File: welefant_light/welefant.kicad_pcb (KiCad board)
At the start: 2 copper layers, 80 x 90 mm, 103 parts, among them J1 Conn_01x02, J2 Conn_02x7_Odd_Even, J3 Conn_02x6_Odd_Even, Q1 AO3401A, Q2 AO3401A, Q3 AO3401A, SW1 ON-OFF, SW2 RESET, SW3 BOOT, SW4 GPIO33, SW5 IO34, U1 RT9080-33GJ5, U2 Audio Jack PJ-324, U3 SD18OB261-060, U4 TP4056, U5 welefant, U6 128MBit Flash, U7 ESP32-S3, U8 Reset 2.8V, X1 40 MHz

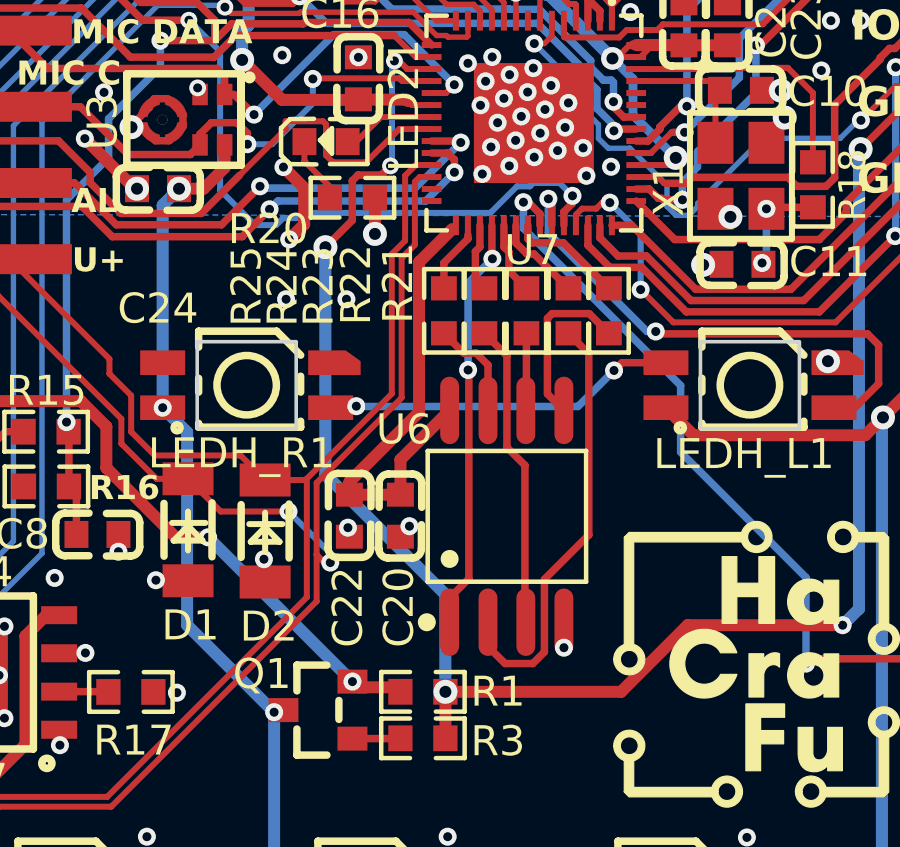
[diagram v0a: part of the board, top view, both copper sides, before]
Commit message: use S3FH4R2 / remove flash chip
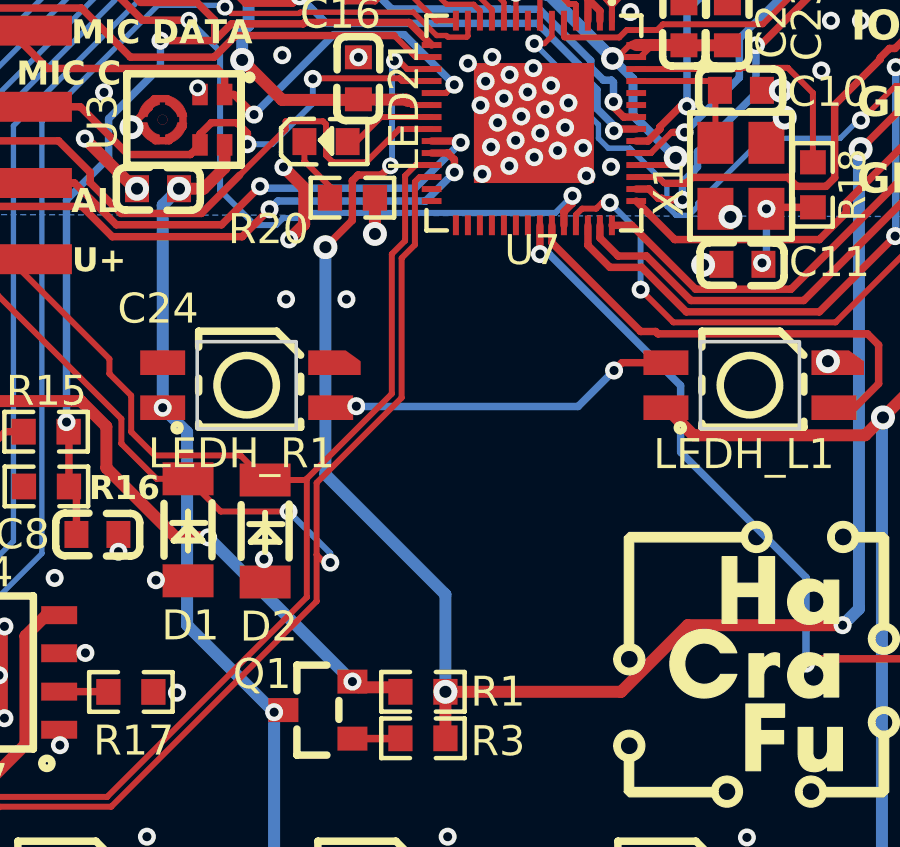
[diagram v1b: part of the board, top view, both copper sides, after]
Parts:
- removed C20: 100n, easyeda2kicad:C0603
- removed C22: 1u, easyeda2kicad:C0603
- removed R21, R22, R23, R24, R25: 0, easyeda2kicad:R0603
- removed U6: 128MBit Flash, easyeda2kicad:SOIC-8_L5.3-W5.3-P1.27-LS8.0-BL
- U7: value ESP32-S3 -> ESP32-S3FH4R2
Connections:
- U7 pad 29: /VDD_SPI -> unconnected-(U7-VDD_SPI-Pad29)
- U7 pad 30: Net-(U7-SPIHD) -> unconnected-(U7-SPIHD-Pad30)
- U7 pad 31: Net-(U7-SPIWP) -> unconnected-(U7-SPIWP-Pad31)
- U7 pad 32: /SPICS0 -> unconnected-(U7-SPICS0-Pad32)
- U7 pad 33: Net-(U7-SPICLK) -> unconnected-(U7-SPICLK-Pad33)
- U7 pad 34: Net-(U7-SPIQ) -> unconnected-(U7-SPIQ-Pad34)
- U7 pad 35: Net-(U7-SPID) -> unconnected-(U7-SPID-Pad35)
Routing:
- net /VDD_SPI: track 15.6 -> 0.00 mm
- net /SPIQ: track 14.6 -> 0.00 mm
- net /SPICS0: track 13.8 -> 0.00 mm, vias 2 -> 0
- net /SPIWP: track 10.2 -> 0.00 mm
- net /SPID: track 5.68 -> 0.00 mm
- net Net-(U7-SPID): track 3.84 -> 0.00 mm
- net /SPIHD: track 3.42 -> 0.00 mm
- net Net-(U7-SPIQ): track 2.96 -> 0.00 mm
- net /SPICLK: track 2.58 -> 0.00 mm
- net Net-(U7-SPICLK): track 2.41 -> 0.00 mm
- net Net-(U7-SPIWP): track 2.29 -> 0.00 mm
- net Net-(U7-SPIHD): track 2.12 -> 0.00 mm
- net /LED_MATRIX: track 35.7 -> 33.8 mm
- net /LED_HEAD: track 17.7 -> 16.0 mm, vias 2 -> 0
- net GND: vias 458 -> 455

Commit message: Revert "use S3FH4R2 / remove flash chip"
This reverts commit b0f4cc23a485e26b2c676c6cda33926215215541.
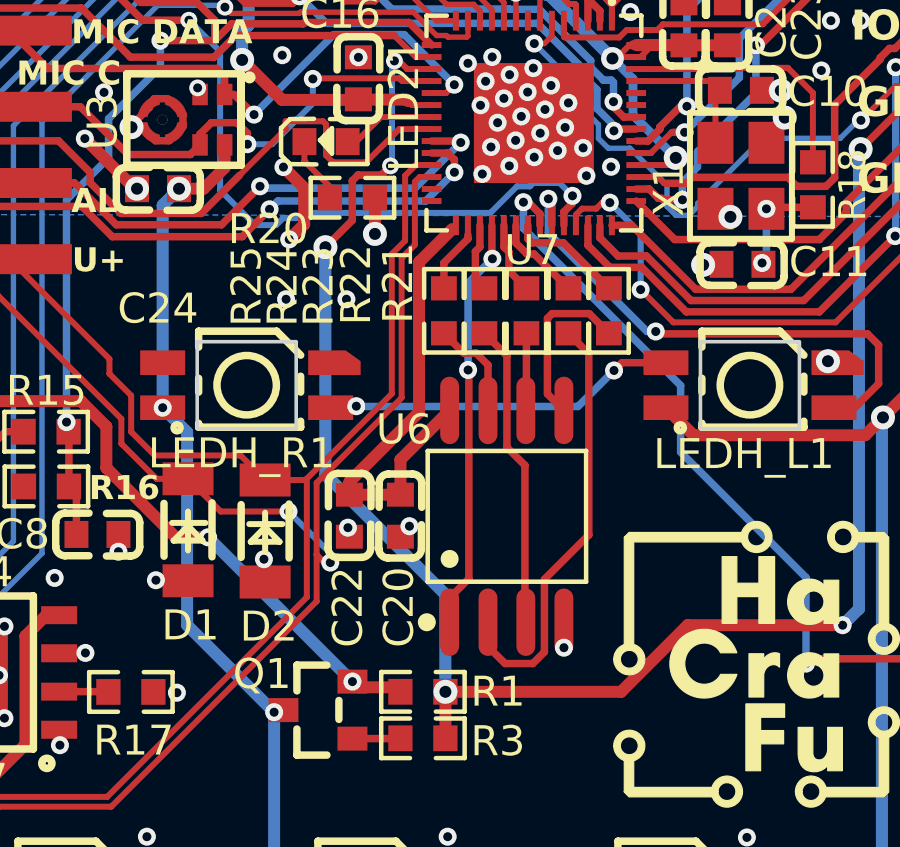
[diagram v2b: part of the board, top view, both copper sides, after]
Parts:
- added C20: 100n, easyeda2kicad:C0603, F.Cu at (68.3, 70.3)
- added C22: 1u, easyeda2kicad:C0603, F.Cu at (66.7, 70.3)
- added R21: 0, easyeda2kicad:R0603, F.Cu at (75.3, 63.5)
- added R22: 0, easyeda2kicad:R0603, F.Cu at (74.0, 63.5)
- added R23: 0, easyeda2kicad:R0603, F.Cu at (72.5, 63.5)
- added R24: 0, easyeda2kicad:R0603, F.Cu at (71.2, 63.5)
- added R25: 0, easyeda2kicad:R0603, F.Cu at (69.8, 63.5)
- added U6: 128MBit Flash, easyeda2kicad:SOIC-8_L5.3-W5.3-P1.27-LS8.0-BL, F.Cu at (71.9, 70.4)
- U7: value ESP32-S3FH4R2 -> ESP32-S3
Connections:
- U7 pad 29: unconnected-(U7-VDD_SPI-Pad29) -> /VDD_SPI
- U7 pad 30: unconnected-(U7-SPIHD-Pad30) -> Net-(U7-SPIHD)
- U7 pad 31: unconnected-(U7-SPIWP-Pad31) -> Net-(U7-SPIWP)
- U7 pad 32: unconnected-(U7-SPICS0-Pad32) -> /SPICS0
- U7 pad 33: unconnected-(U7-SPICLK-Pad33) -> Net-(U7-SPICLK)
- U7 pad 34: unconnected-(U7-SPIQ-Pad34) -> Net-(U7-SPIQ)
- U7 pad 35: unconnected-(U7-SPID-Pad35) -> Net-(U7-SPID)
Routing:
- net /VDD_SPI: track 0.00 -> 15.6 mm
- net /SPIQ: track 0.00 -> 14.6 mm
- net /SPICS0: track 0.00 -> 13.8 mm, vias 0 -> 2
- net /SPIWP: track 0.00 -> 10.2 mm
- net /SPID: track 0.00 -> 5.68 mm
- net Net-(U7-SPID): track 0.00 -> 3.84 mm
- net /SPIHD: track 0.00 -> 3.42 mm
- net Net-(U7-SPIQ): track 0.00 -> 2.96 mm
- net /SPICLK: track 0.00 -> 2.58 mm
- net Net-(U7-SPICLK): track 0.00 -> 2.41 mm
- net Net-(U7-SPIWP): track 0.00 -> 2.29 mm
- net Net-(U7-SPIHD): track 0.00 -> 2.12 mm
- net /LED_MATRIX: track 33.8 -> 35.7 mm
- net /LED_HEAD: track 16.0 -> 17.7 mm, vias 0 -> 2
- net GND: vias 455 -> 458
